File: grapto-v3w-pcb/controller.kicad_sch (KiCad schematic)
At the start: 50 parts, among them J1 Conn_01x06_Female, J2 USB_C_Receptacle_USB2.0, J3 USB_C_Receptacle_USB2.0, U1 MAX17260TFDN, U2 MCP7383x-2xMC, U3 AP9211S-AL, U4 USBLC6-4SC6, U5 ACN52840, U6 TPS2110, U7 LM3676SD-3.3

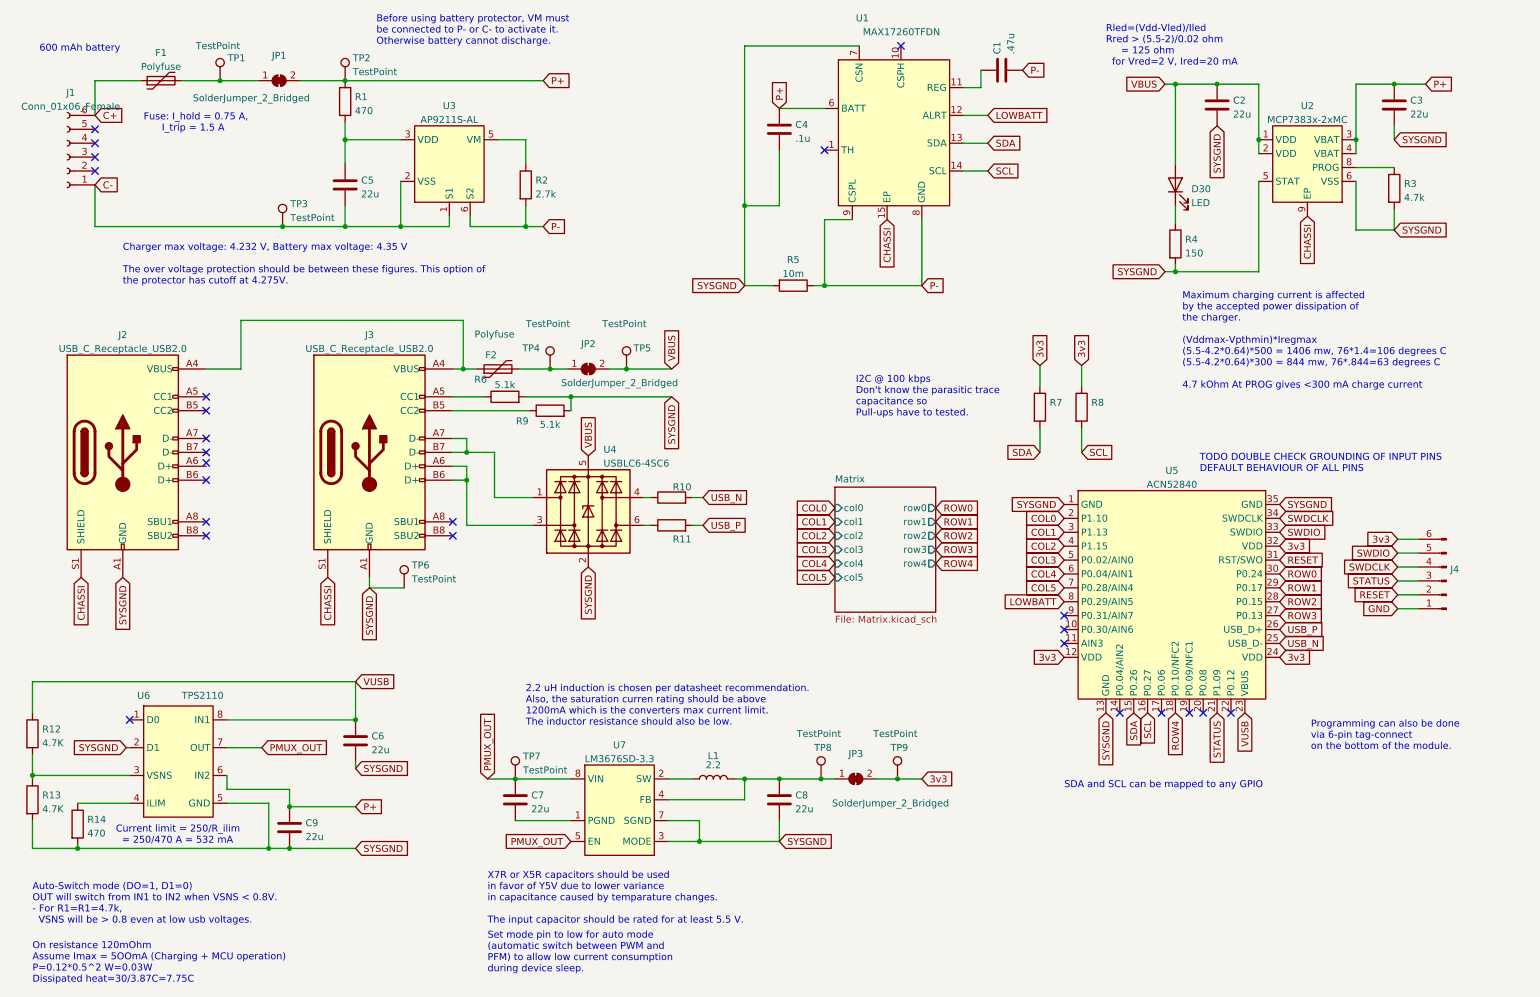
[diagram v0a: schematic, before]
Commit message: Footprints done.
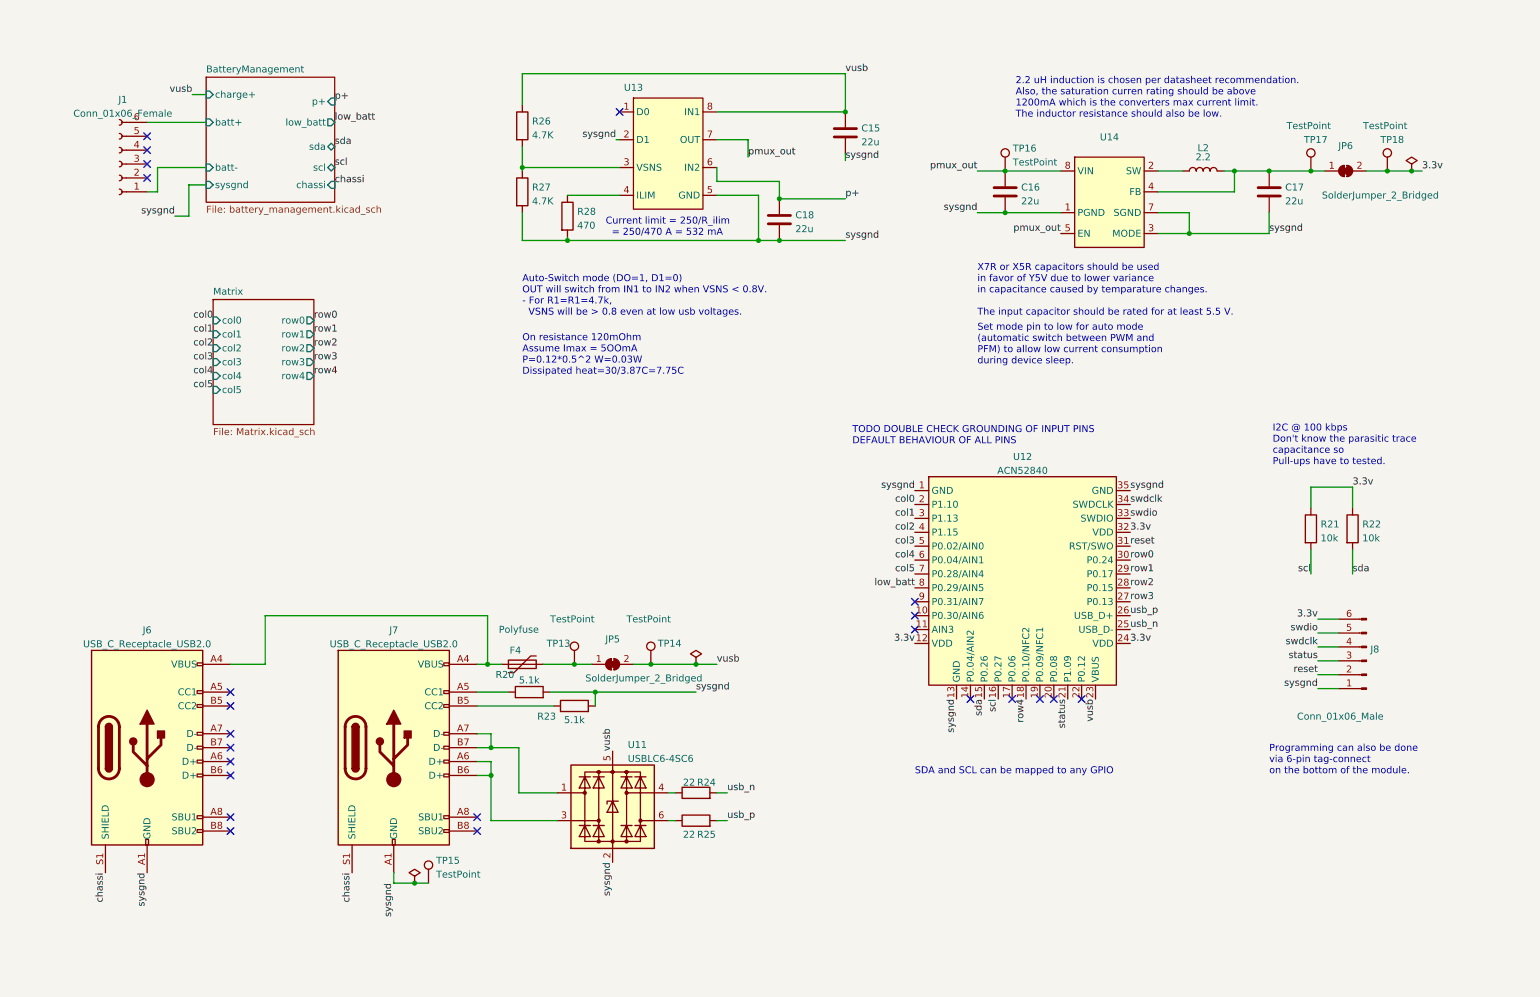
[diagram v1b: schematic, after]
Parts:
- removed C1: .47u, symbol Device:C
- removed C2, C3, C5: 22u, symbol Device:C
- removed C4: .1u, symbol Device:C
- removed D30: LED, symbol Device:LED
- removed F1: Polyfuse, symbol Device:Polyfuse
- removed JP1: SolderJumper_2_Bridged, symbol Jumper:SolderJumper_2_Bridged
- removed R1: 470, symbol Device:R
- removed R2: 2.7k, symbol Device:R
- removed R3: 4.7k, symbol Device:R
- removed R4: 150, symbol Device:R
- removed R5: 10m, symbol Device:R
- removed TP1, TP2, TP3: TestPoint, symbol Connector:TestPoint
- removed U1: MAX17260TFDN, symbol grapto-v3w:MAX17260TFDN
- removed U2: MCP7383x-2xMC, symbol grapto-v3w:MCP7383x-2xMC
- removed U3: AP9211S-AL, symbol grapto-v3w:AP9211S-AL
- J8: renamed from J4; value (none) -> Conn_01x06_Male
- R21: renamed from R7; value (none) -> 10k
- R22: renamed from R8; value (none) -> 10k
- R24: renamed from R10; value (none) -> 22
- R25: renamed from R11; value (none) -> 22
- U13: renamed from U6; value TPS2110 -> (none)
- U14: renamed from U7; value LM3676SD-3.3 -> (none)
- renumbered C6 to C15, C7 to C16, C8 to C17, C9 to C18, F2 to F4, J2 to J6, J3 to J7, JP2 to JP5, JP3 to JP6, L1 to L2, R6 to R20, R9 to R23, R12 to R26, R13 to R27, R14 to R28, TP4 to TP13, TP5 to TP14, TP6 to TP15, TP7 to TP16, TP8 to TP17, TP9 to TP18, U4 to U11, U5 to U12
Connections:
- net GND is gone; now on net sysgnd: J8.1 (Pin_1)
- net SYSGND is gone; now on net sysgnd: C15.2, C17.2, C18.2, J6.A1 (GND), J6.A12 (GND), J6.B1 (GND), J6.B12 (GND), J7.A1 (GND), J7.A12 (GND), J7.B1 (GND), J7.B12 (GND), R20.2, R23.2, R27.2, R28.2, TP15.1, U11.2 (GND), U12.1 (GND), U12.13 (GND), U12.35 (GND), U13.2 (D1), U13.5 (GND), U14.3 (MODE), U14.7 (SGND)
- net VUSB is gone; now on net vusb: C15.1, R26.1, U12.23 (VBUS), U13.8 (IN1)
- net sysgnd: now reaches C16.2, U14.1 (PGND)
- net 3v3 renamed 3.3v
- net C+ renamed BatteryManagement/batt+
- net C- renamed BatteryManagement/batt-
- net CHASSI renamed chassi
- net COL0 renamed col0
- net COL1 renamed col1
- net COL2 renamed col2
- net COL3 renamed col3
- net COL4 renamed col4
- net COL5 renamed col5
- net LOWBATT renamed low_batt
- net P+ renamed p+
- net PMUX_OUT renamed pmux_out
- net RESET renamed reset
- net ROW0 renamed row0
- net ROW1 renamed row1
- net ROW2 renamed row2
- net ROW3 renamed row3
- net ROW4 renamed row4
- net SCL renamed scl
- net scl: now also R21.2; no longer R22.2
- net SDA renamed sda
- net sda: now also R22.2; no longer R21.2
- net STATUS renamed status
- net SWDCLK renamed swdclk
- net SWDIO renamed swdio
- net USB_N renamed usb_n
- net USB_P renamed usb_p
- net VBUS renamed vusb
- no-connect marks 25 -> 23
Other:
- added sheet BatteryManagement (battery_management.kicad_sch)
- note added: "On resistance 120mOhm Assume Imax = 5OOmA P=0.12*0.5^2 W=0.03W Dissipated heat=30/3.87C=7.75C"
- note removed: "600 mAh battery"
- note removed: "Before using battery protector, VM must be connected to P- or C- to activate it. Otherwise battery cannot discharge."
- note removed: "Charger max voltage: 4.232 V, Battery max voltage: 4.35 V The over voltage protection should be between these figures. This option of the protector has cutoff at 4.275V."
- note removed: "Fuse: I_hold = 0.75 A, I_trip = 1.5 A"
- note removed: "Maximum charging current is affected by the accepted power dissipation of the charger. (Vddmax-Vpthmin)*Iregmax (5.5-4.2*0.64)*500 = 1406 mw, 76*1.4=106 degrees C (5.5-4.2*0.64)*300 = 844 mw, 76*.844=63 degrees C 4.7 kOhm At PROG gives <300 mA charge current"
- note removed: "On resistance 120mOhm Assume Imax = 5OOmA (Charging + MCU operation) P=0.12*0.5^2 W=0.03W Dissipated heat=30/3.87C=7.75C"
- note removed: "Rled=(Vdd-Vled)/Iled Rred > (5.5-2)/0.02 ohm = 125 ohm for Vred=2 V, Ired=20 mA"
- moved on the sheet: C15, C16, C17, C18, F4, J6, J7, J8, JP5, JP6, L2, R20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
